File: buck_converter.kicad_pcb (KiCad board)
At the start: 2 copper layers, 67.3 x 21.5 mm, 17 parts, among them J1 Screw_Terminal_01x02, J2 Screw_Terminal_01x02

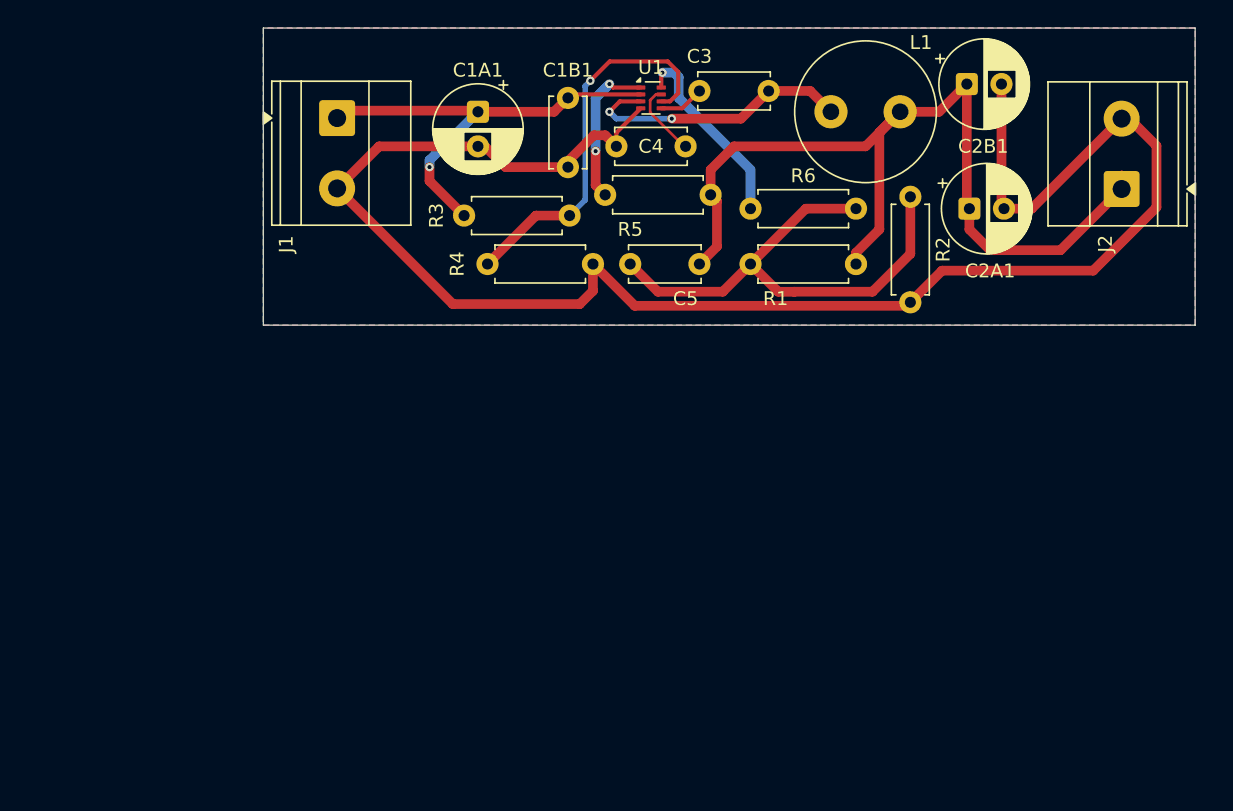
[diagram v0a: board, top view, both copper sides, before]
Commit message: Fixed
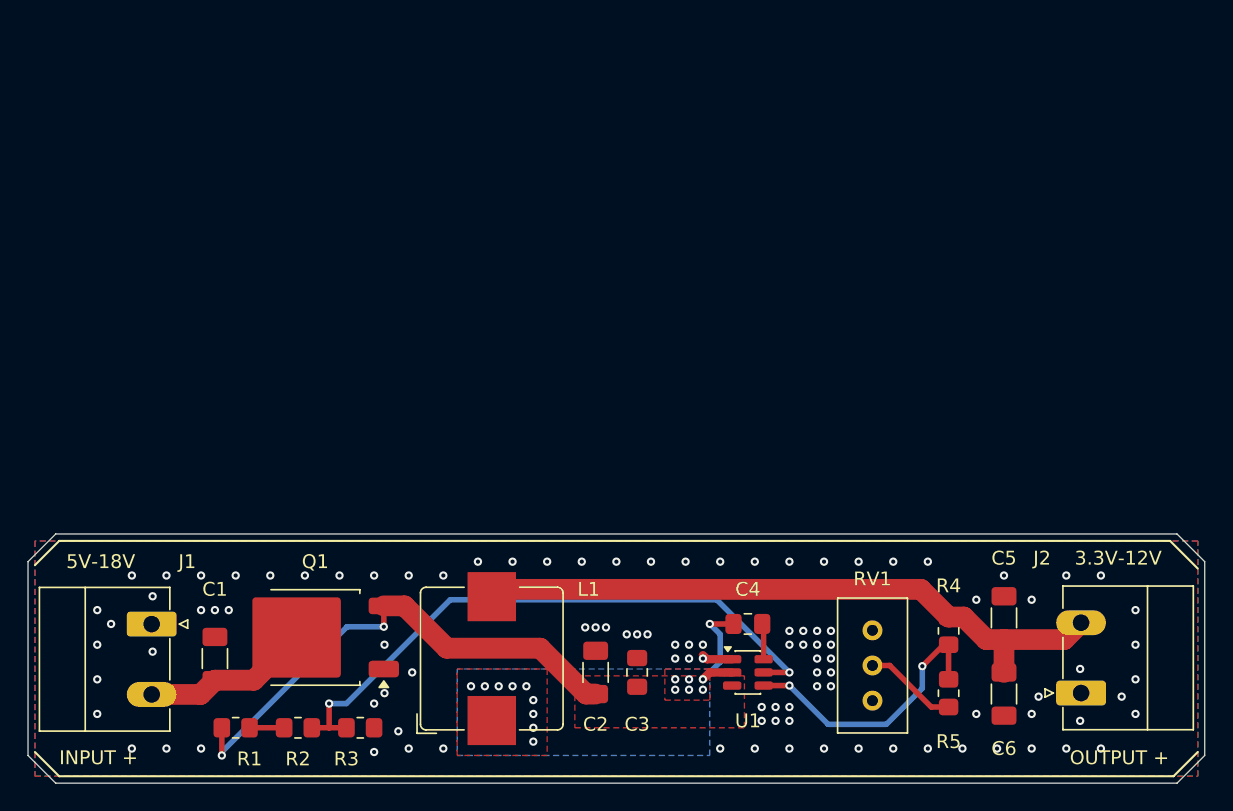
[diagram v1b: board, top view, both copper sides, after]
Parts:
- removed C1A1, C2A1, C2B1: 22uF, Capacitor_THT:CP_Radial_D6.3mm_P2.50mm
- removed C1B1: 0.1uF, Capacitor_THT:C_Disc_D5.0mm_W2.5mm_P5.00mm
- removed R6: 10k, Resistor_THT:R_Axial_DIN0207_L6.3mm_D2.5mm_P7.62mm_Horizontal
- added C1: 22u, Capacitor_SMD:C_1206_3216Metric_Pad1.33x1.80mm_HandSolder, F.Cu at (123.5, 106.0)
- added C2: 22u, Capacitor_SMD:C_1206_3216Metric_Pad1.33x1.80mm_HandSolder, F.Cu at (151.0, 107.0)
- added C6: 22u, Capacitor_SMD:C_1206_3216Metric_Pad1.33x1.80mm_HandSolder, F.Cu at (180.5, 108.6)
- added Q1: SUD09P10-195, Package_TO_SOT_SMD:TO-252-2, F.Cu at (130.7, 104.5)
- added RV1: 20K, Potentiometer_THT:Potentiometer_Bourns_3296W_Vertical, F.Cu at (171.0, 104.0)
- C3: value 0.1uF -> 100n; footprint Capacitor_THT:C_Disc_D5.0mm_W2.5mm_P5.00mm -> Capacitor_SMD:C_0805_2012Metric_Pad1.18x1.45mm_HandSolder
- C4: value 22nF -> 100n; footprint Capacitor_THT:C_Disc_D5.0mm_W2.5mm_P5.00mm -> Capacitor_SMD:C_0805_2012Metric_Pad1.18x1.45mm_HandSolder
- C5: value 300pF -> 22u; footprint Capacitor_THT:C_Disc_D5.0mm_W2.5mm_P5.00mm -> Capacitor_SMD:C_1206_3216Metric_Pad1.33x1.80mm_HandSolder
- J1: value Screw_Terminal_01x02 -> Input Screw Terminal; footprint TerminalBlock_Phoenix:TerminalBlock_Phoenix_MKDS-1,5-2-5.08_1x02_P5.08mm_Horizontal -> Connector_Phoenix_MC_HighVoltage:PhoenixContact_MC_1,5_2-G-5.08_1x02_P5.08mm_Horizontal
- J2: value Screw_Terminal_01x02 -> Output Screw Terminal; footprint TerminalBlock_Phoenix:TerminalBlock_Phoenix_MKDS-1,5-2-5.08_1x02_P5.08mm_Horizontal -> Connector_Phoenix_MC_HighVoltage:PhoenixContact_MC_1,5_2-G-5.08_1x02_P5.08mm_Horizontal
- L1: value 6.6uH -> 15u; footprint Inductor_THT:L_Radial_D10.0mm_P5.00mm_Neosid_SD12k_style3 -> Inductor_SMD:L_Bourns_SRP1038C_10.0x10.0mm
- R1: value 90.9k -> 100K; footprint Resistor_THT:R_Axial_DIN0207_L6.3mm_D2.5mm_P7.62mm_Horizontal -> Resistor_SMD:R_0805_2012Metric_Pad1.20x1.40mm_HandSolder
- R2: value 10k -> 100K; footprint Resistor_THT:R_Axial_DIN0207_L6.3mm_D2.5mm_P7.62mm_Horizontal -> Resistor_SMD:R_0805_2012Metric_Pad1.20x1.40mm_HandSolder
- R3: value 191k -> 100K; footprint Resistor_THT:R_Axial_DIN0207_L6.3mm_D2.5mm_P7.62mm_Horizontal -> Resistor_SMD:R_0805_2012Metric_Pad1.20x1.40mm_HandSolder
- R4: value 49.9k -> 100K; footprint Resistor_THT:R_Axial_DIN0207_L6.3mm_D2.5mm_P7.62mm_Horizontal -> Resistor_SMD:R_0805_2012Metric_Pad1.20x1.40mm_HandSolder
- R5: value 10k -> 5K; footprint Resistor_THT:R_Axial_DIN0207_L6.3mm_D2.5mm_P7.62mm_Horizontal -> Resistor_SMD:R_0805_2012Metric_Pad1.20x1.40mm_HandSolder
- U1: value ~ -> TPS54308; footprint Package_TO_SOT_SMD:SOT-583-8 -> Package_TO_SOT_SMD:SOT-23-6
- moved R2 58.5 mm to (129.5, 111.0), turned to 0 degrees
- moved R1 50.1 mm to (125.0, 111.0)
- moved L1 46.5 mm to (143.5, 106.0), turned to 90 degrees
- moved R5 43.7 mm to (176.5, 108.5), turned to -90 degrees
- moved R4 42.6 mm to (176.5, 104.0), turned to -90 degrees
- moved C3 42.2 mm to (154.0, 107.0), turned to 90 degrees
- moved U1 42.1 mm to (162.0, 107.0)
- moved J1 38.9 mm to (118.9, 103.5)
- moved R3 37.8 mm to (134.0, 111.0)
- moved C5 37.2 mm to (180.5, 103.1), turned to 90 degrees
- moved J2 36.5 mm to (186.1, 108.5)
- moved C4 34.8 mm to (162.0, 103.5)
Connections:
- C3 pad 1: Net-(U1-BST) -> /VIN_P
- C3 pad 2: Net-(U1-SW) -> GND
- C4 pad 1: Net-(U1-SS) -> Net-(U1-BOOT)
- C4 pad 2: GND -> /SW
- C5 pad 1: Net-(C5-Pad1) -> /VOUT
- C5 pad 2: VOUT -> GND
- J1 pad 1: 24V -> GND
- J1 pad 2: GND -> /VIN
- J2 pad 1: VOUT -> GND
- J2 pad 2: GND -> /VOUT
- L1 pad 1: Net-(U1-SW) -> /SW
- L1 pad 2: VOUT -> /VOUT
- R1 pad 1: Net-(C5-Pad1) -> /VIN_P
- R1 pad 2: VOUT -> Net-(R1-Pad2)
- R2 pad 1: Net-(C5-Pad1) -> Net-(R1-Pad2)
- R2 pad 2: GND -> /EN
- R3 pad 1: 24V -> /EN
- R3 pad 2: Net-(U1-EN) -> GND
- R4 pad 1: Net-(U1-EN) -> /VOUT
- R4 pad 2: GND -> /FB
- R5 pad 1: Net-(U1-PG) -> /FB
- R5 pad 2: VOUT -> Net-(R5-Pad2)
- U1 pad 1: Net-(U1-PG) -> GND
- U1 pad 2: 24V -> /SW
- U1 pad 3: Net-(U1-SW) -> /VIN_P
- U1 pad 4: GND -> /FB
- U1 pad 5: Net-(U1-BST) -> /EN
- U1 pad 6: Net-(U1-EN) -> Net-(U1-BOOT)
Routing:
- net GND: track 125.0 -> 2.24 mm, vias 0 -> 104
- net VOUT: track 66.2 -> 0.00 mm
- net /VOUT: track 0.00 -> 47.4 mm
- net /EN: track 0.00 -> 44.6 mm, vias 0 -> 2
- net Net-(C5-Pad1): track 37.3 -> 0.00 mm
- net /VIN_P: track 0.00 -> 36.6 mm, vias 0 -> 2
- net 24V: track 32.7 -> 0.00 mm, vias 1 -> 0
- net Net-(U1-EN): track 28.0 -> 0.00 mm, vias 1 -> 0
- net Net-(U1-SW): track 20.5 -> 0.00 mm, vias 2 -> 0
- net /FB: track 0.00 -> 20.3 mm, vias 0 -> 2
- net Net-(U1-FB): track 14.1 -> 0.00 mm, vias 1 -> 0
- net /VIN: track 0.00 -> 12.2 mm
- net Net-(U1-PG): track 11.1 -> 0.00 mm, vias 2 -> 0
- net /SW: track 0.00 -> 8.86 mm, vias 0 -> 16
- net Net-(R5-Pad2): track 0.00 -> 6.74 mm
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- added copper zone on B.Cu, net /SW
- added copper zone on F.Cu, net /SW
- added copper zone on F.Cu, net /VIN_P
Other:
- board size 67.3 x 21.5 mm -> 85 x 18 mm
- board text added: "3.3V-12V"
- board text added: "3A Buck Converter"
- board text added: "5V-18V"
- board text added: "INPUT +"
- board text added: "OUTPUT +"
